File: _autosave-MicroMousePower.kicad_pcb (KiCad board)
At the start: 2 copper layers, 58.6 x 55 mm, 104 parts, among them J1 USB_C_Receptacle_PowerOnly_6P, J2 Conn_02x16_Odd_Even, J3 Conn_01x02_Pin, Q1 TIP41C, Q2 TIP41C, Q3 TIP41C, U1 INA219AxDCN, U2 MCP73831-3-MC, U3 CH224K, U4 DRV8833PWPR, U5 DRV8833PWPR, U6 TPS61023DRLR, U8 AP62300WU, U9 TC1262-33

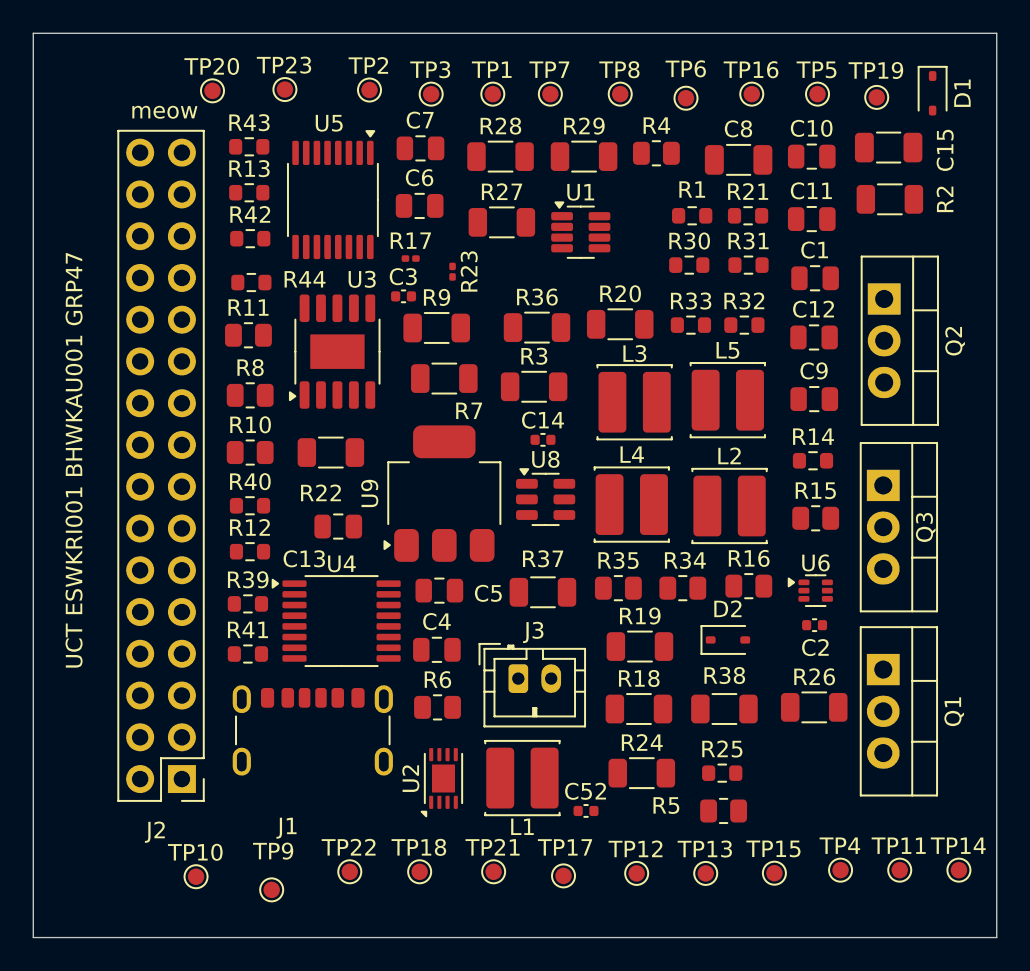
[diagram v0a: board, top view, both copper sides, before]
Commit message: there is light at the end
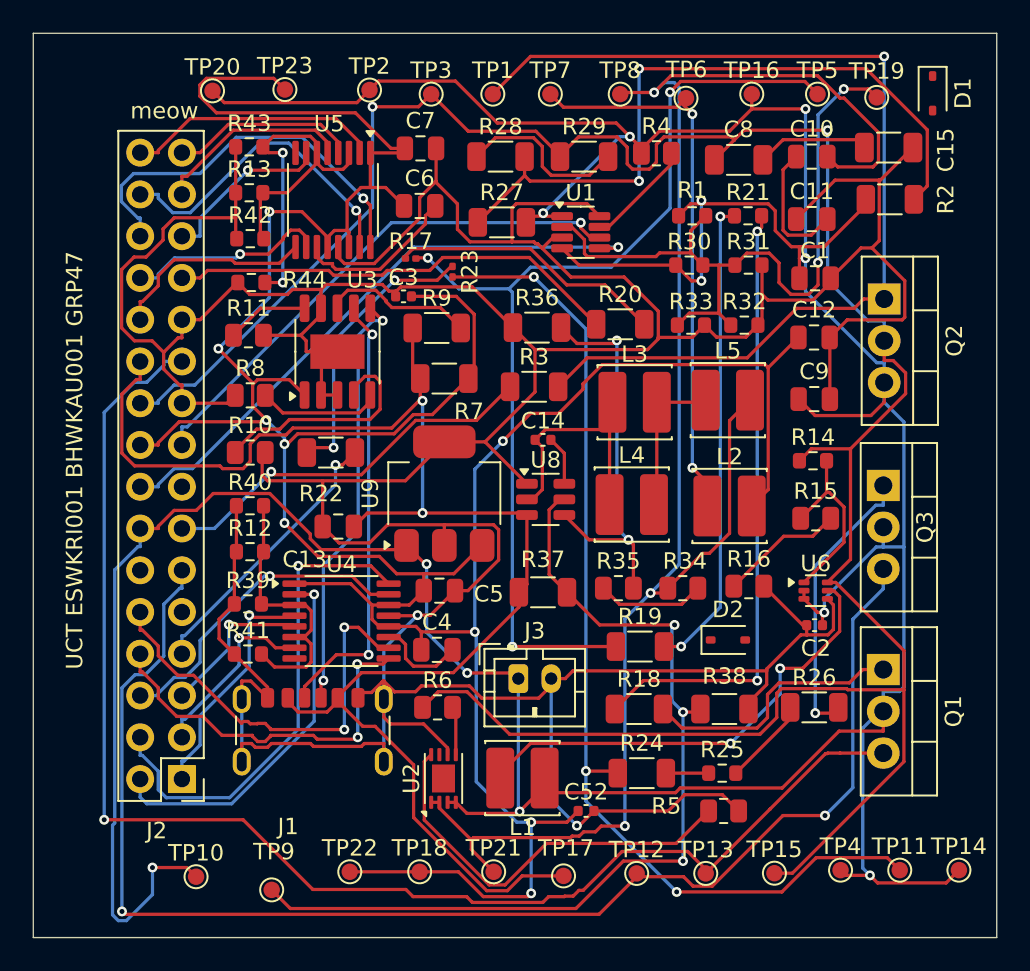
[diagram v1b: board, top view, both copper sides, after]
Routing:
- net -BATT: track 0.00 -> 324.7 mm, vias 0 -> 2
- net +BATT: track 0.00 -> 262.3 mm, vias 0 -> 12
- net /3V3: track 0.00 -> 199.9 mm, vias 0 -> 9
- net /5V: track 0.00 -> 152.6 mm, vias 0 -> 2
- net /USB 5V: track 0.00 -> 101.8 mm, vias 0 -> 3
- net /9V: track 0.00 -> 93.5 mm, vias 0 -> 2
- net /EXT_LOAD1_OUT: track 0.00 -> 85.3 mm, vias 0 -> 1
- net /EXT_LOAD2_OUT: track 0.00 -> 85.2 mm, vias 0 -> 2
- net Net-(D1-PadC): track 0.00 -> 63.0 mm, vias 0 -> 3
- net Net-(D2-PadC): track 0.00 -> 62.7 mm, vias 0 -> 3
- net Net-(Q2-B): track 0.00 -> 61.5 mm, vias 0 -> 1
- net Net-(U8-EN): track 0.00 -> 56.5 mm, vias 0 -> 3
- net Net-(U1-IN-): track 0.00 -> 43.7 mm, vias 0 -> 2
- net Net-(R2-Pad1): track 0.00 -> 42.7 mm, vias 0 -> 2
- net Net-(R18-Pad1): track 0.00 -> 37.8 mm, vias 0 -> 2
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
